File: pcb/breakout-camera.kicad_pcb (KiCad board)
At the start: 2 copper layers, 38.1 x 39.4 mm, 36 parts, among them P10 CONN_01X14, P4 CONN_01X04, P5 CONN_01X01, Q1 2SC5095, Q2 MT3S20TU, Q3 2SC5095, Q4 MT3S20TU, U10 ICX825AQA, U4 TXB0104, U9 CXD3400N

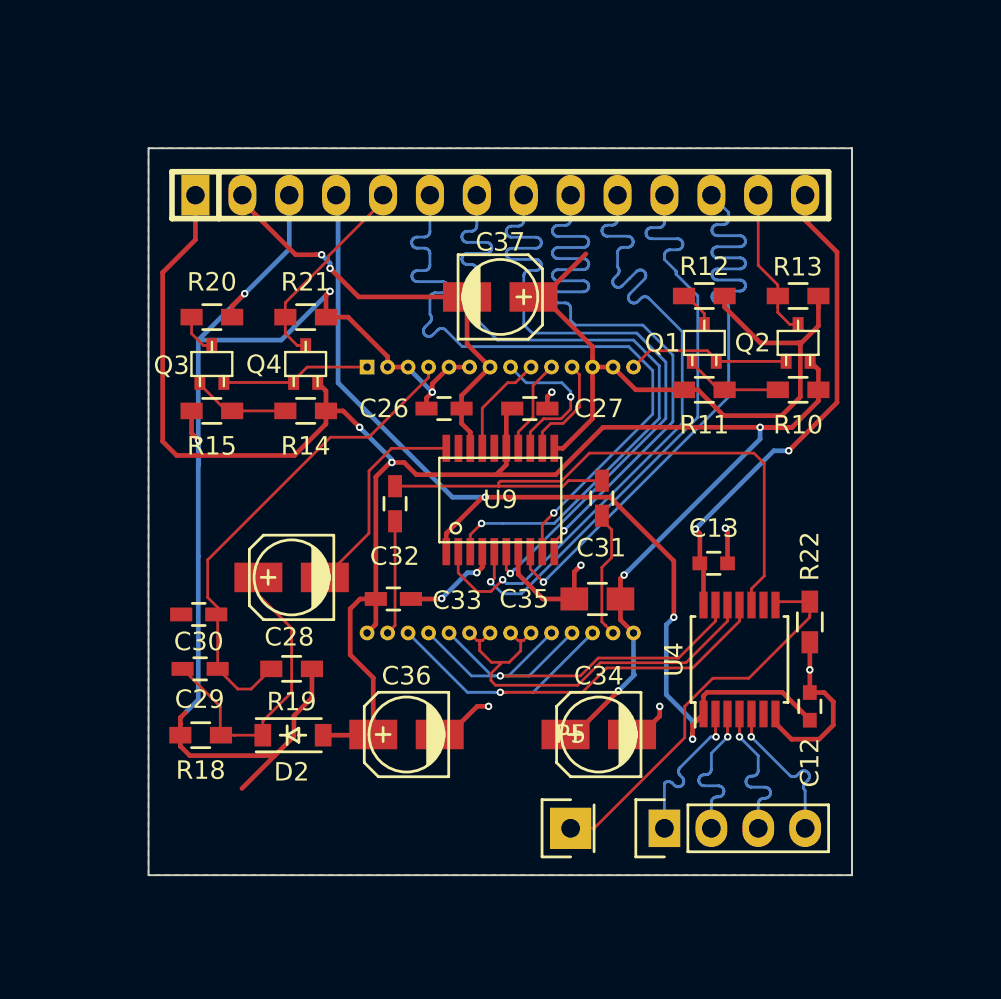
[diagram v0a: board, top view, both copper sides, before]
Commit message: More work
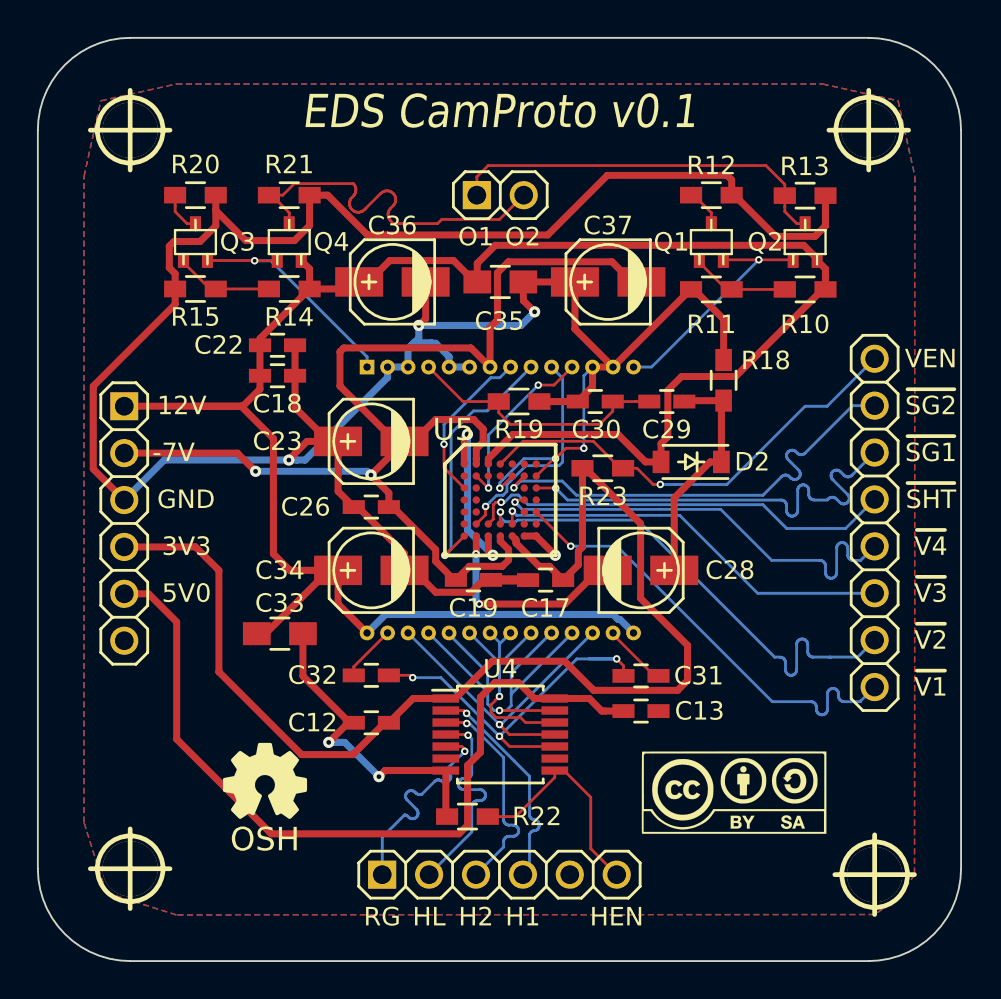
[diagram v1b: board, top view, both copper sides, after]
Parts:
- removed C27: 0.1u, Capacitors_SMD:C_0603_HandSoldering
- removed P4: CONN_01X04, Socket_Strips:Socket_Strip_Straight_1x04
- removed P5: CONN_01X01, Socket_Strips:Socket_Strip_Straight_1x01
- removed U9: CXD3400N, w_smd_dil:tssop-20
- added C17: 0.1uF, Capacitors_SMD:C_0603_HandSoldering, F.Cu at (78.7, 67.8)
- added C18: 0.1uF/25V, Capacitors_SMD:C_0603_HandSoldering, F.Cu at (64.1, 56.8)
- added C19: 0.1uF/10V, Capacitors_SMD:C_0603_HandSoldering, F.Cu at (74.7, 67.8)
- added C22: 1.0uF/25V, Capacitors_SMD:C_0603_HandSoldering, F.Cu at (64.1, 55.1)
- added C23: 4.7uF/10V, Capacitors_SMD:c_elec_4x5.3, F.Cu at (69.2, 60.3)
- added G***: LOGO, w_logo:Logo_silk_CC-BY-SA_10x4.5mm, F.Cu at (88.9, 79.3)
- added Horizontal: HORI, xess:HDR_1x6, F.Cu at (76.2, 83.8)
- added P6: POWER, xess:HDR_1x6, F.Cu at (55.8, 64.8)
- added P7: VERT, xess:xess-1X08, F.Cu at (96.5, 64.7)
- added R23: 10.0k, Resistors_SMD:R_0603_HandSoldering, F.Cu at (81.7, 61.8)
- added REF**: OSH, xess:oshw-logo2, F.Cu at (63.5, 78.7)
- added U5: ADDI9023, engstad:csp-bga-bc-40-1, F.Cu at (76.2, 63.5)
- added hole_3mm: VAL**, w_details:hole_3mm, F.Cu at (96.5, 83.8)
- added hole_3mm: VAL**, w_details:hole_3mm, F.Cu at (56.2, 83.5)
- added hole_3mm: VAL**, w_details:hole_3mm, F.Cu at (56.2, 43.5)
- added hole_3mm: VAL**, w_details:hole_3mm, F.Cu at (96.2, 43.5)
- C12, C13: footprint Capacitors_SMD:C_0603 -> Capacitors_SMD:C_0603_HandSoldering
- C33: footprint Capacitors_SMD:C_0603_HandSoldering -> Capacitors_SMD:C_0805_HandSoldering
- P10: value CONN_01X14 -> OUTP; footprint w_pin_strip:pin_strip_14 -> xess:HDR_1x2
- U10: footprint camera:ICX825 -> sony:icx-825
- moved R18 34.2 mm to (88.3, 57.0), turned to 90 degrees
- moved C29 29.1 mm to (85.2, 58.2), turned to 180 degrees
- moved D2 26.2 mm to (86.5, 61.4), turned to 180 degrees
- moved C36 24.5 mm to (70.4, 51.7)
- moved C30 24.4 mm to (81.3, 58.2)
- moved C12 23.8 mm to (69.2, 75.6), turned to 180 degrees
- moved R22 21.3 mm to (74.4, 80.6), turned to 180 degrees
- moved R19 19.0 mm to (77.2, 58.2)
- moved C28 18.9 mm to (83.8, 67.3), turned to 0 degrees
- moved C35 18.0 mm to (76.2, 51.7), turned to 180 degrees
- moved C34 15.2 mm to (69.2, 67.3)
- moved U4 13.6 mm to (76.2, 76.2), turned to 0 degrees
- moved C31 9.86 mm to (83.8, 73.0), turned to 180 degrees
- moved C32 9.38 mm to (69.2, 73.0), turned to 0 degrees
- moved C13 8.92 mm to (83.8, 74.9)
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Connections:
- net /camera/H1S_1 renamed /camera/OH1
- net /camera/H2S_1 renamed /camera/OH2
- net /camera/LH1_1 renamed /camera/OLH
- net Net-(C28-Pad1) renamed /camera/SCKP
- C28 pad 2: Net-(C28-Pad2) -> /camera/SUBCK
- P10 pad 1: /camera/12V -> /camera/CCD_OUT1
- P10 pad 2: /camera/-7V -> /camera/CCD_OUT2
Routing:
- net GND: track 140.8 -> 191.1 mm, vias 12 -> 11
- net /camera/-7V: track 25.0 -> 65.0 mm
- net /camera/VDREN: track 0.00 -> 24.6 mm, vias 0 -> 1
- net /camera/5V0: track 26.7 -> 43.8 mm, vias 2 -> 0
- net /camera/XV3: track 38.1 -> 22.2 mm
- net /camera/XSHT: track 38.1 -> 23.4 mm
- net /camera/ORG: track 34.7 -> 21.3 mm, vias 0 -> 3
- net /camera/XV1: track 38.4 -> 25.0 mm
- net /camera/XV4: track 38.1 -> 24.7 mm
- net /camera/XSGV3: track 38.1 -> 24.9 mm
- net /camera/CCD_OUT1: track 8.16 -> 21.2 mm
- net /camera/SUB: track 26.6 -> 14.4 mm
- net /camera/SUBCK: track 0.00 -> 11.5 mm, vias 0 -> 2
- net Net-(C28-Pad2): track 11.4 -> 0.00 mm
- net /camera/OLH: track 28.3 -> 17.3 mm
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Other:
- board size 38.1 x 39.4 mm -> 50 x 50 mm
- net class Power: trace_width 0.254 -> 0.381; via_dia 0.4064 -> 0.6096; via_drill 0.2032 -> 0.4064
- board text added: "-7V"
- board text added: "12V"
- board text added: "3V3"
- board text added: "5V0"
- board text added: "EDS CamProto v0.1"
- board text added: "GND"
- board text added: "H1"
- board text added: "H2"
- board text added: "HEN"
- board text added: "HL"
- board text added: "O1"
- board text added: "O2"
- board text added: "RG"
- board text added: "SG1"
- board text added: "SG2"
- board text added: "SHT"
- board text added: "V1"
- board text added: "V2"
- board text added: "V3"
- board text added: "V4"
- board text added: "VEN"
